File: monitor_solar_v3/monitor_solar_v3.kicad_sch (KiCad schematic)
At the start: 41 parts, among them J1 Panel, J10 GPIO, J11 Jumper, J2 ACS712, J3 Battery, J4 AMP_OUT, J5 JUMPER_PROG, J6 JUMPER_PROG, J7 PROGRAM, J9 Reg 5V, SW1 SW_Push, U1 LM7805_TO220, U2 AMS1117-3.3, U3 ESP-12F, U4 LM358, U5 4051

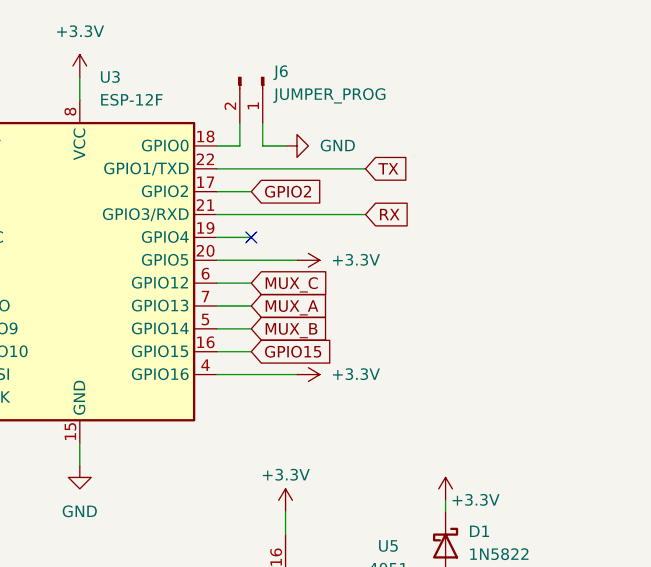
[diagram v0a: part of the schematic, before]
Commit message: PCB V3 finished
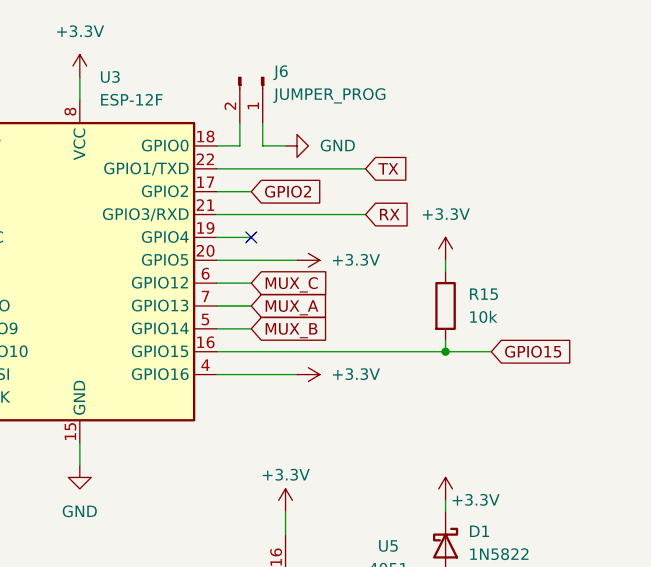
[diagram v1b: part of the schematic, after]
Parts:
- added R15: 10k, Resistor_THT:R_Axial_DIN0207_L6.3mm_D2.5mm_P10.16mm_Horizontal, symbol Device:R
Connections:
- net +3.3V: now also R15.1
- net GPIO15: now also R15.2
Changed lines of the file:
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@@
 	)
 	(junction
+		(at 260.35 60.96)
+		(diameter 0)
+		(color 0 0 0 0)
+	)
+	(junction
 		(at 22.86 25.4)
 		(diameter 0)
@@
 	(wire
 		(pts
+			(xy 260.35 50.8) (xy 260.35 52.07)
+		)
+		(stroke
+			(width 0)
+			(type default)
+		)
+	)
+	(wire
+		(pts
 			(xy 49.53 134.62) (xy 49.53 132.08)
 		)
@@
 	(wire
 		(pts
-			(xy 238.76 60.96) (xy 234.95 60.96)
-		)
-		(stroke
-			(width 0)
-			(type default)
-		)
-	)
-	(wire
-		(pts
 			(xy 48.26 81.28) (xy 50.8 81.28)
 		)
@@
 	(wire
 		(pts
+			(xy 260.35 60.96) (xy 234.95 60.96)
+		)
+		(stroke
+			(width 0)
+			(type default)
+		)
+	)
+	(wire
+		(pts
 			(xy 196.85 25.4) (xy 199.39 25.4)
 		)
@@
 	(wire
 		(pts
+			(xy 260.35 59.69) (xy 260.35 60.96)
+		)
+		(stroke
+			(width 0)
+			(type default)
+		)
+	)
+	(wire
+		(pts
 			(xy 196.85 151.13) (xy 186.69 151.13)
 		)
@@
 	(wire
 		(pts
+			(xy 260.35 60.96) (xy 265.43 60.96)
+		)
+		(stroke
+			(width 0)
+			(type default)
+		)
+	)
+	(wire
+		(pts
 			(xy 22.86 45.72) (xy 25.4 45.72)
 		)
@@
 	(global_label "GPIO15"
 		(shape input)
-		(at 238.76 60.96 0)
+		(at 265.43 60.96 0)
 		(fields_autoplaced yes)
 		(effects
@@
 		)
 		(property "Intersheetrefs" "${INTERSHEET_REFS}"
-			(at 248.6395 60.96 0)
+			(at 275.3095 60.96 0)
 			(effects
 				(font
@@
 	)
 	(symbol
+		(lib_id "power:+3.3V")
+		(at 260.35 50.8 0)
+		(unit 1)
+		(exclude_from_sim no)
+		(in_bom yes)
+		(on_board yes)
+		(dnp no)
+		(fields_autoplaced yes)
+		(property "Reference" "#PWR034"
+			(at 260.35 54.61 0)
+			(effects
+				(font
+					(size 1.27 1.27)
+				)
+				(hide yes)
+			)
+		)
+		(property "Value" "+3.3V"
+			(at 260.35 45.72 0)
+			(effects
+				(font
+					(size 1.27 1.27)
+				)
+			)
+		)
+		(property "Footprint" ""
+			(at 260.35 50.8 0)
+			(effects
+				(font
+					(size 1.27 1.27)
+				)
+				(hide yes)
+			)
+		)
+		(property "Datasheet" ""
+			(at 260.35 50.8 0)
+			(effects
+				(font
+					(size 1.27 1.27)
+				)
+				(hide yes)
+			)
+		)
+		(property "Description" "Power symbol creates a global label with name \"+3.3V\""
+			(at 260.35 50.8 0)
+			(effects
+				(font
+					(size 1.27 1.27)
+				)
+				(hide yes)
+			)
+		)
+		(pin "1"
+		)
+		(instances
+			(project "monitor_solar_v3"
+				(path "/d4e2a079-328a-41d5-a5a0-7716b5883be5"
+					(reference "#PWR034")
+					(unit 1)
+				)
+			)
+		)
+	)
+	(symbol
 		(lib_id "power:GND")
 		(at 186.69 156.21 0)
@@
 					(unit 1)
 				)
+			)
+		)
+	)
+	(symbol
+		(lib_id "Device:R")
+		(at 260.35 55.88 0)
+		(unit 1)
+		(exclude_from_sim no)
+		(in_bom yes)
+		(on_board yes)
+		(dnp no)
+		(fields_autoplaced yes)
+		(property "Reference" "R15"
+			(at 262.89 54.6099 0)
+			(effects
+				(font
+					(size 1.27 1.27)
+				)
+				(justify left)
+			)
+		)
+		(property "Value" "10k"
+			(at 262.89 57.1499 0)
+			(effects
+				(font
+					(size 1.27 1.27)
+				)
+				(justify left)
+			)
+		)
+		(property "Footprint" "Resistor_THT:R_Axial_DIN0207_L6.3mm_D2.5mm_P10.16mm_Horizontal"
+			(at 258.572 55.88 90)
+			(effects
+				(font
+					(size 1.27 1.27)
+				)
+				(hide yes)
+			)
+		)
+		(property "Datasheet" "~"
+			(at 260.35 55.88 0)
+			(effects
+				(font
+					(size 1.27 1.27)
+				)
+				(hide yes)
+			)
+		)
+		(property "Description" "Resistor"
+			(at 260.35 55.88 0)
+			(effects
+				(font
+					(size 1.27 1.27)
+				)
+				(hide yes)
+			)
+		)
+		(pin "1"
+		)
+		(pin "2"
+		)
+		(instances
+			(project "monitor_solar_v3"
+				(path "/d4e2a079-328a-41d5-a5a0-7716b5883be5"
+					(reference "R15")
+					(unit 1)
+				)
